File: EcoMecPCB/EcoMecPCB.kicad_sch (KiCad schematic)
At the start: 43 parts, among them J10 MPU-6050, J11 LC, J2 Encoder, J3 Conn_01x02_Pin, J4 Conn_01x02_Pin, J5 Conn_01x03_Pin, J6 Conn_01x02_Pin, J7 Conn_01x03_Pin, U1 CS1237-SO, U2 MT2492, U3 SIT65HVD230DR, U4 AZ1117-3.3, U5 TL431ACDBZR, U6 STM32F_dev

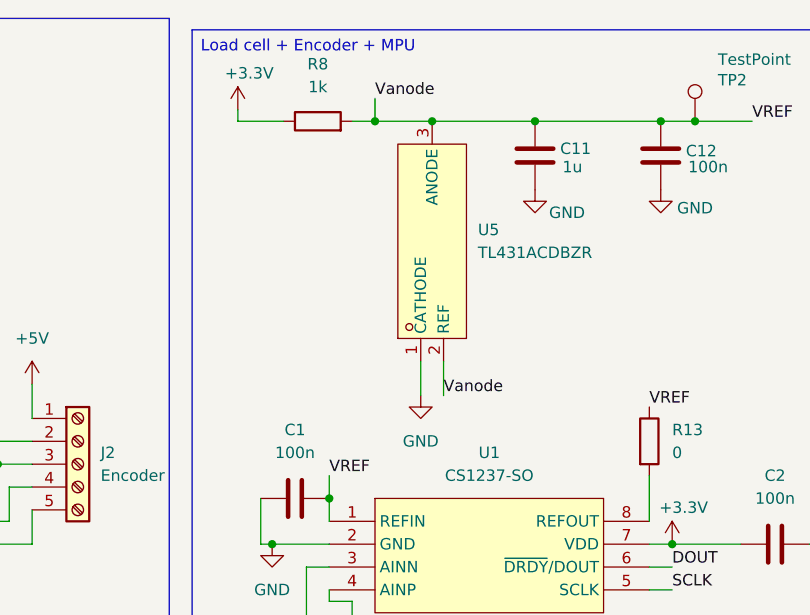
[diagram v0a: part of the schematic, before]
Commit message: Update
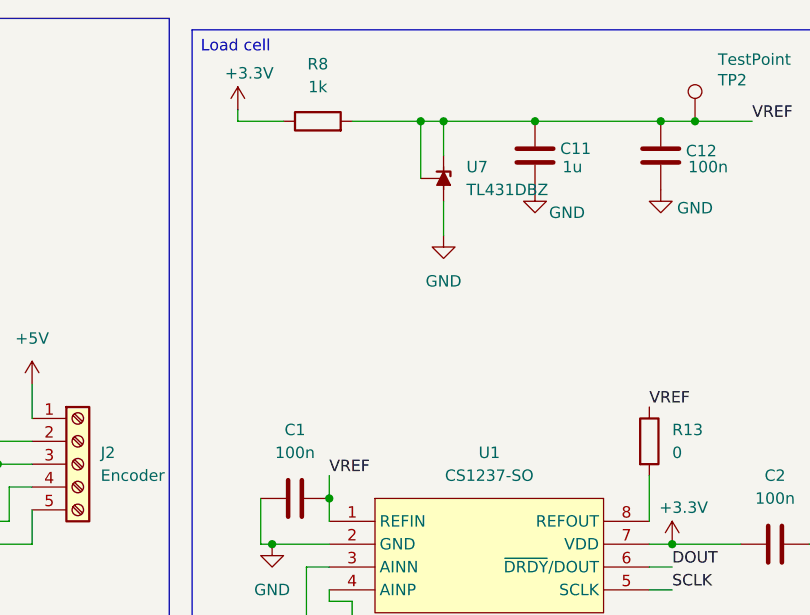
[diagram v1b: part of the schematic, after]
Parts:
- removed U5: TL431ACDBZR, EasyEDA:SOT-23-3_L3.0-W1.7-P0.95-LS2.9-BR, symbol EasyEDA:TL431ACDBZR
- added U7: TL431DBZ, Package_TO_SOT_SMD:SOT-23, symbol Reference_Voltage:TL431DBZ
- C1, C10, C11, C12, C2, C8, C9: footprint (none) -> Capacitor_SMD:C_1206_3216Metric_Pad1.33x1.80mm_HandSolder
- C3, C4, C5, C6, C7: footprint LED_SMD:LED_1206_3216Metric_Pad1.42x1.75mm_HandSolder -> Capacitor_SMD:C_1206_3216Metric_Pad1.33x1.80mm_HandSolder
- J10: footprint (none) -> Connector_PinHeader_2.54mm:PinHeader_1x08_P2.54mm_Vertical
- J11: footprint (none) -> TerminalBlock_Phoenix:TerminalBlock_Phoenix_PT-1,5-4-3.5-H_1x04_P3.50mm_Horizontal
- J2: footprint (none) -> TerminalBlock_Phoenix:TerminalBlock_Phoenix_PT-1,5-5-3.5-H_1x05_P3.50mm_Horizontal
- R10, R11, R12, R13, R6, R7, R8, R9: footprint (none) -> Resistor_SMD:R_1206_3216Metric_Pad1.30x1.75mm_HandSolder
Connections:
- net GND: now also U7.3 (A)
- net VREF: now also U7.1 (K), U7.2 (REF)
